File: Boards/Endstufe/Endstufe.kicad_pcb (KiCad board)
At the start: 2 copper layers, 55 parts, among them P1 CONN_3, P2 Trafo, P3 Relais, P4 6V3_AC, P5 Trafo_GK, P6 6V3_DC, P7 VSup1, P9 VSup3, T1 KT88, T2 KT88, U1 ECC82, U2 ECC83

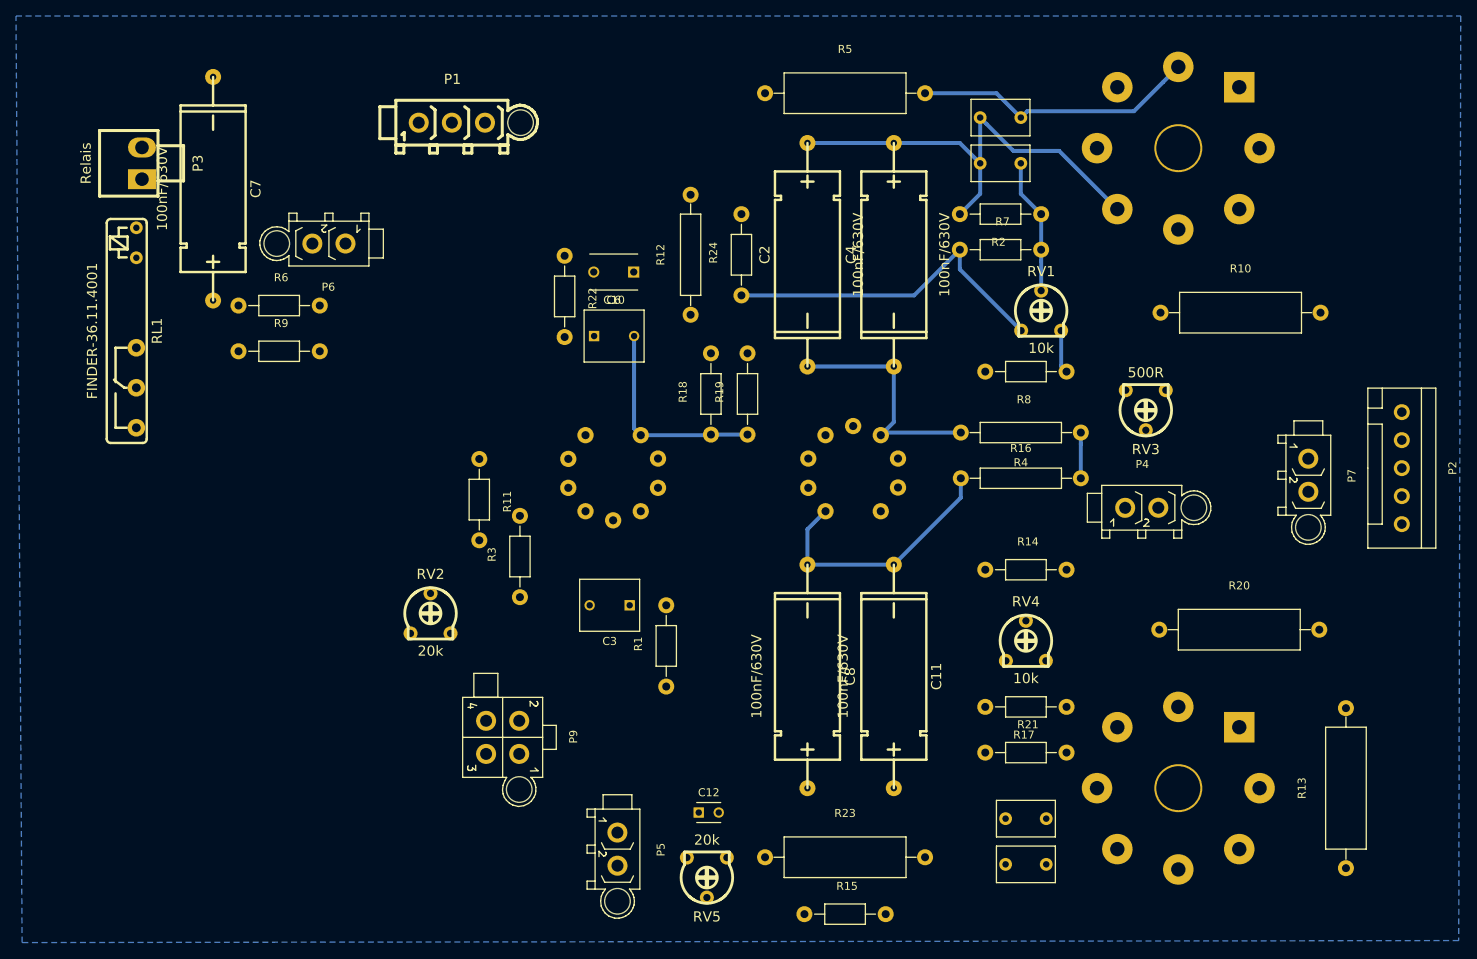
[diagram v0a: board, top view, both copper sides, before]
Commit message: Work in Progress
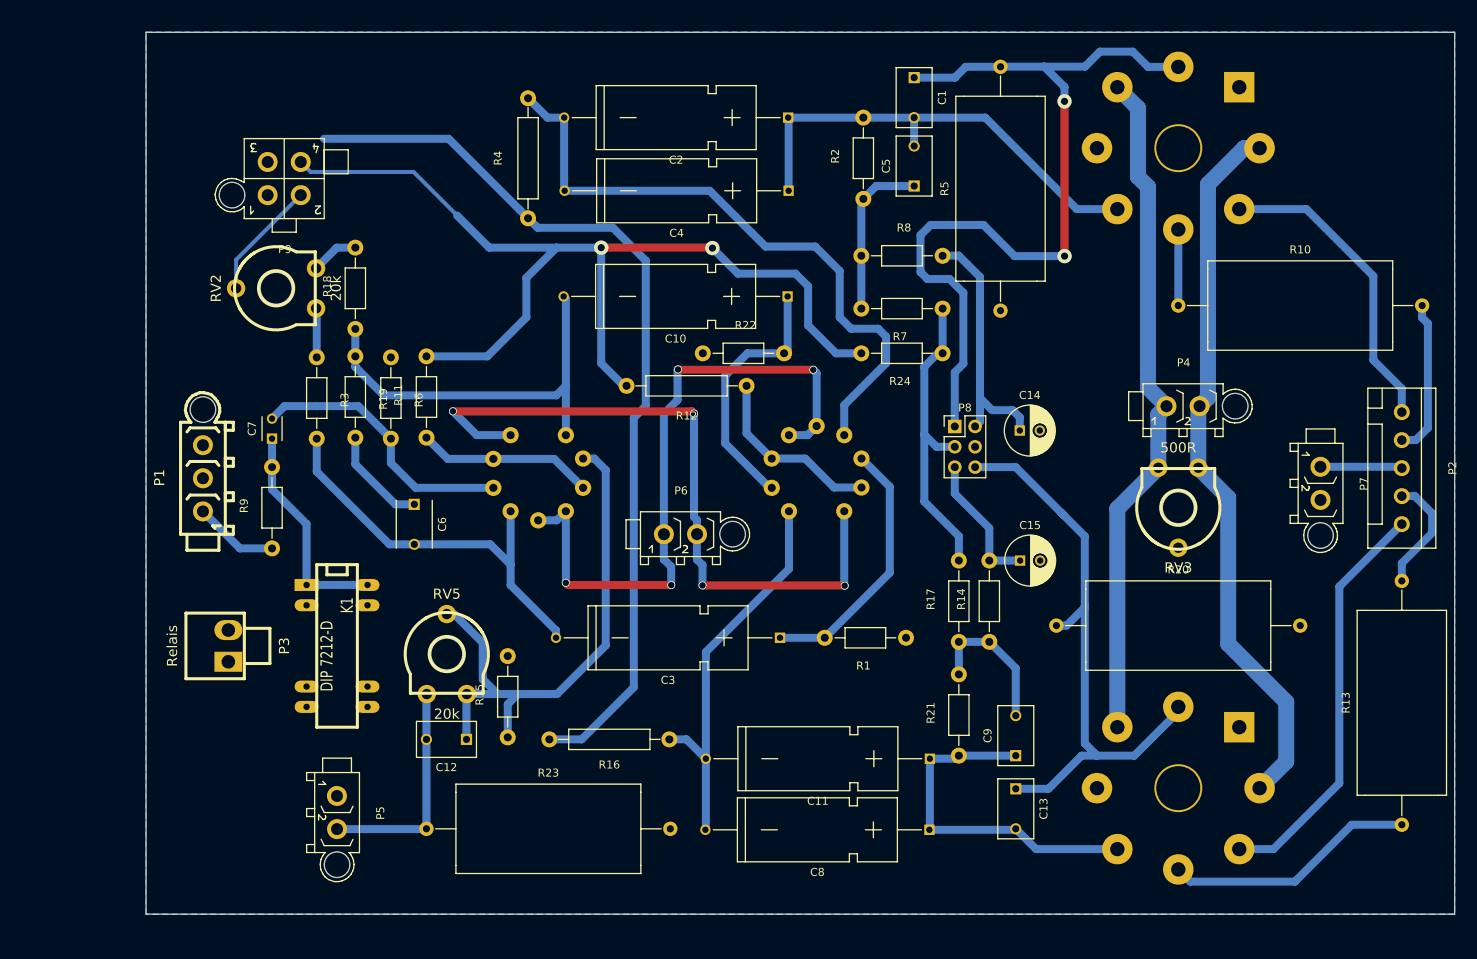
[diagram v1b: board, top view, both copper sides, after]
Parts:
- removed RL1: FINDER-36.11.4001, w_relay:relay_34.51
- removed RV1, RV4: 10k, w_pth_resistors:trimmer_piher_pt6xv
- added C14: 10µF / 100V, Capacitors_ThroughHole:C_Radial_D6.3_L11.2_P2.5, F.Cu at (158.0, 101.6)
- added C15: 10µF / 100V, Capacitors_ThroughHole:C_Radial_D6.3_L11.2_P2.5, F.Cu at (158.0, 117.9)
- added K1: DIP 7212-D, Reed:REED, F.Cu at (72.6, 128.5)
- added P8: Bias, Pin_Headers:Pin_Header_Straight_2x03_Pitch2.54mm, F.Cu at (149.9, 101.1)
- C1, C13, C5, C9: value 68pF -> 68pF / 500V; footprint Capacitor-Wima-FKP2-630v:Capacitor-Wima-FKP2-630v-R5B4K5 -> Capacitors_ThroughHole:C_Disc_D7.5_P5
- C10, C3: value 100nF -> 100nF / 400V; footprint Capacitors_ThroughHole:C_Rect_L7.5_W6.5_P5 -> Capacitors_ThroughHole:C_Axial_D8_L21_P28
- C11, C2, C4, C8: value 100nF/630V -> 100nF/400V; footprint w_capacitors:CPA_8x21MM -> Capacitors_ThroughHole:C_Axial_D8_L21_P28
- C12: value 100pF -> 100pF / 500V; footprint Capacitors_ThroughHole:C_Disc_D3_P2.5 -> Capacitors_ThroughHole:C_Disc_D7.5_P5
- C6: value 33pF -> 33pF / 500V
- C7: value 100nF/630V -> 100nF; footprint w_capacitors:CPA_8x21MM -> Capacitors_ThroughHole:C_Disc_D3_P2.5
- R10, R13, R20, R23, R5: footprint Resistors_ThroughHole:Resistor_Horizontal_RM20mm -> Resistors_ThroughHole:Resistor_Ceramic_Horizontal_L23mm-W9mm-H9mm-p30mm
- R24: value 1M -> 30k
- R9: value 68k -> 220R
- RV2, RV3, RV5: footprint w_pth_resistors:trimmer_piher_pt6xv -> w_pth_resistors:trimmer_piher_pt10xv10
- moved P9 75.0 mm to (66.0, 70.1), turned to 180 degrees
- moved R4 70.5 mm to (96.5, 67.6), turned to 90 degrees
- moved P3 61.3 mm to (59.1, 128.5)
- moved R16 60.9 mm to (106.7, 140.2), turned to 180 degrees
- moved P6 57.0 mm to (115.6, 114.6), turned to 0 degrees
- moved P1 54.3 mm to (55.9, 107.6), turned to 90 degrees
- moved R15 50.2 mm to (94.0, 134.9), turned to 90 degrees
- moved R19 49.0 mm to (74.9, 97.4), turned to 270 degrees
- moved R18 46.4 mm to (74.9, 83.8)
- moved RV2 45.0 mm to (65.0, 83.8), turned to 270 degrees
- moved RV5 42.9 mm to (86.4, 129.5), turned to 180 degrees
- moved C6 39.9 mm to (82.3, 110.8), turned to 270 degrees
- moved R23 37.3 mm to (99.1, 151.4)
- moved P5 35.3 mm to (72.6, 149.4)
- moved R3 32.2 mm to (70.1, 97.5), turned to 270 degrees
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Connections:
- net Net-(C1-Pad1) renamed Bias_1
- net Net-(C13-Pad1) renamed Bias_2
- C5 pad 1: Net-(C5-Pad1) -> UG_1
- C9 pad 2: Net-(C9-Pad2) -> UG_2
- P1 pad 1: Net-(C7-Pad2) -> Net-(P1-Pad1)
- P9 pad 3: -120V -> GND
- P9 pad 4: GND -> -120V
- R14 pad 1: GND -> UG_2
- R17 pad 1: Net-(C9-Pad2) -> UG_2
- R2 pad 1: Net-(C5-Pad1) -> UG_1
- R21 pad 2: Net-(C9-Pad2) -> UG_2
- R7 pad 2: Net-(C5-Pad1) -> UG_1
- R8 pad 1: Net-(R8-Pad1) -> UG_1
- R8 pad 2: GND -> Net-(C14-Pad1)
- R9 pad 1: Net-(C7-Pad1) -> Net-(P1-Pad1)
- R9 pad 2: Net-(C7-Pad2) -> Net-(C7-Pad1)
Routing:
- net -120V: track 0.00 -> 126.4 mm, vias 0 -> 2
- net +300V: track 5.72 -> 113.8 mm
- net Net-(P4-Pad2): track 0.00 -> 90.2 mm
- net Net-(P6-Pad2): track 0.00 -> 87.7 mm, vias 0 -> 4
- net Net-(P4-Pad1): track 0.00 -> 85.1 mm
- net 6V3: track 0.00 -> 82.3 mm, vias 0 -> 4
- net Bias_2: track 0.00 -> 75.4 mm
- net Bias_1: track 35.5 -> 108.4 mm, vias 0 -> 2
- net Net-(C12-Pad1): track 0.00 -> 70.0 mm
- net Net-(P2-Pad5): track 0.00 -> 51.5 mm
- net Net-(C3-Pad2): track 0.00 -> 51.3 mm
- net Net-(C2-Pad2): track 30.2 -> 80.3 mm
- net Net-(C11-Pad1): track 0.00 -> 44.4 mm
- net Net-(P2-Pad1): track 0.00 -> 38.8 mm
- net Net-(C7-Pad2): track 0.00 -> 34.3 mm
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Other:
- board outline added: 163.6 x 110.2 mm
